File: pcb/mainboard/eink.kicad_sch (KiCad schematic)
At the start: 48 parts, among them J401 FH12-40S-0.5SH, U401 MAX17135

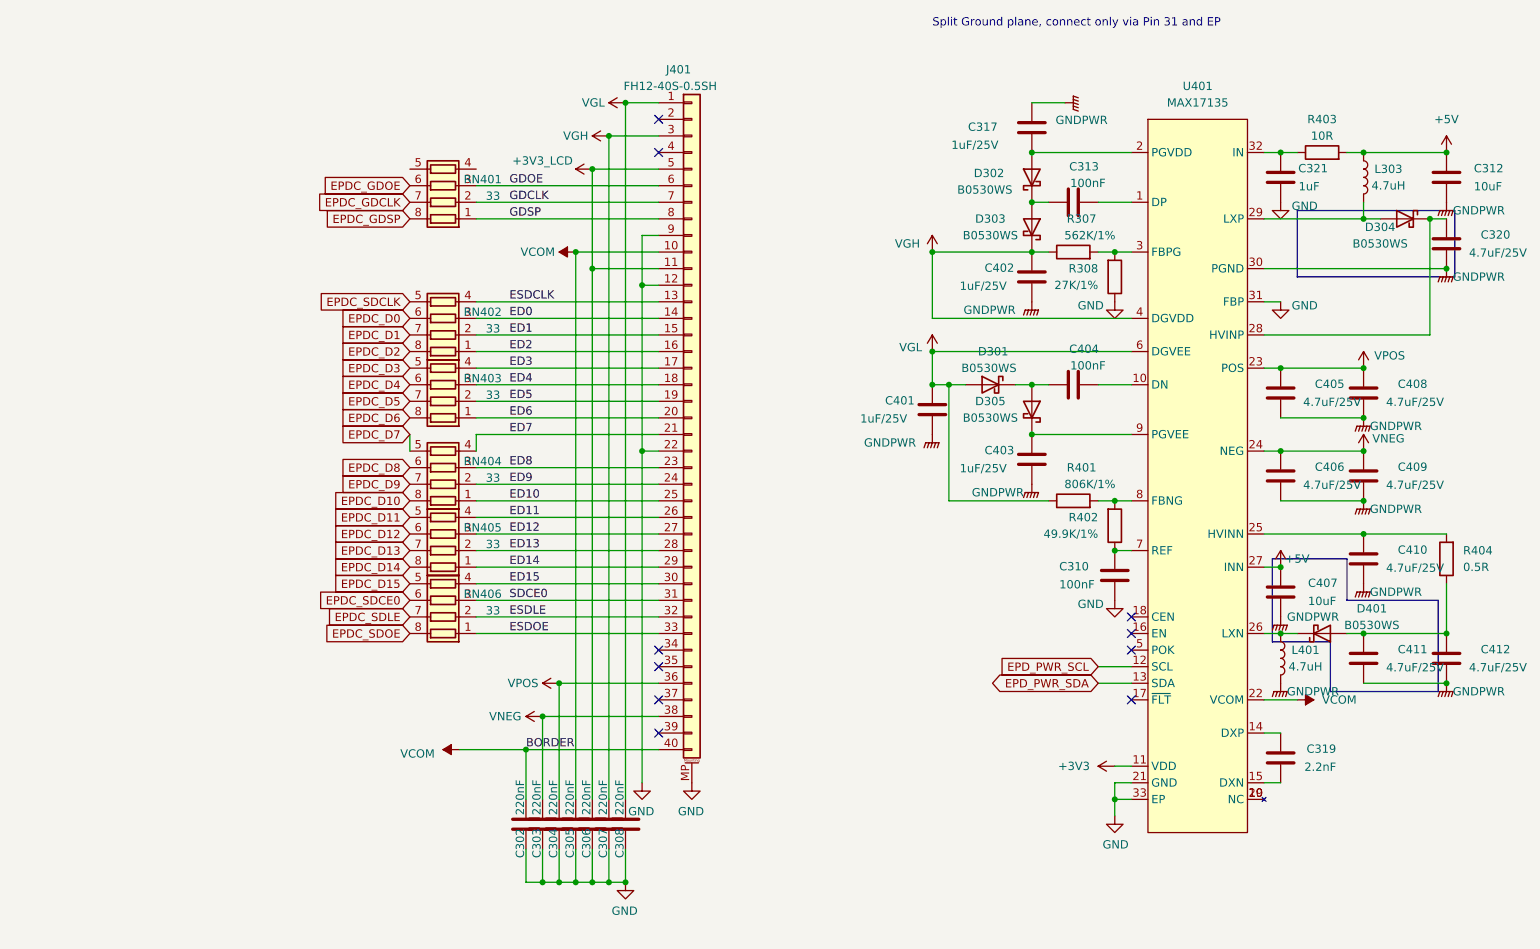
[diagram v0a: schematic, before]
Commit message: pcb: r0p4
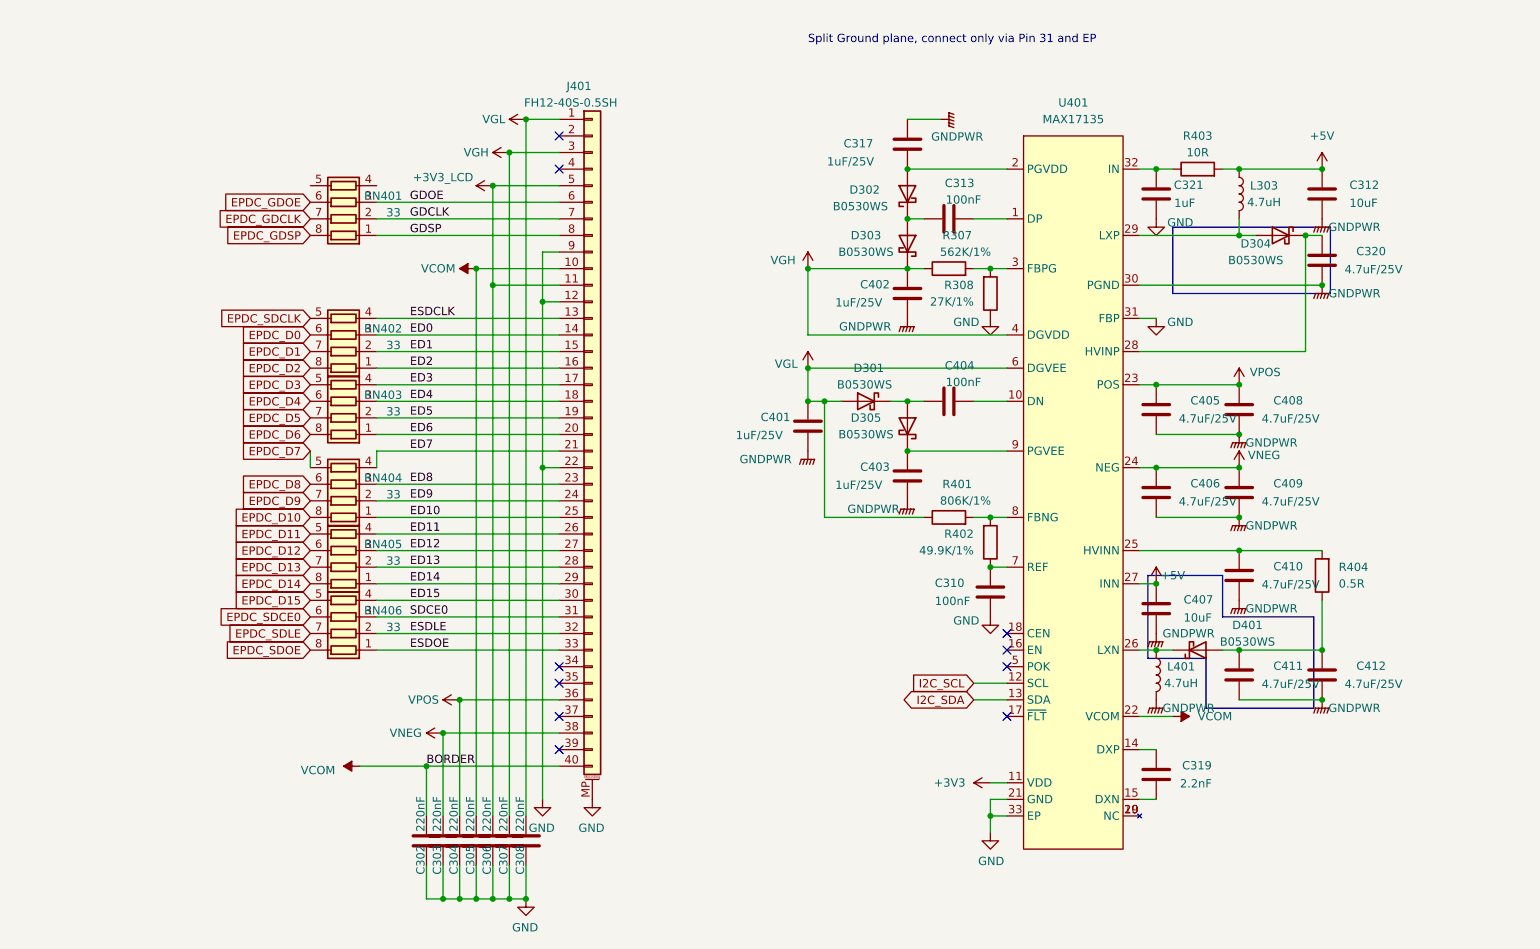
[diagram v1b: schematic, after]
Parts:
- L303, L401: footprint footprints:L_1212 -> footprints:L_FXL0420; LCSC C340379 -> C167208
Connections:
- net EPD_PWR_SCL renamed I2C_SCL
- net EPD_PWR_SDA renamed I2C_SDA
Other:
- company: Copyright 2021 Modos / Engineer: Wenting Zhang -> Copyright 2022 Modos / Engineer: Wenting Zhang
- moved on the sheet: C302, C303, C304, C305, C306, C307, C308, C310, C312, C313, C317, C319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

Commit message: pcb: r0p5
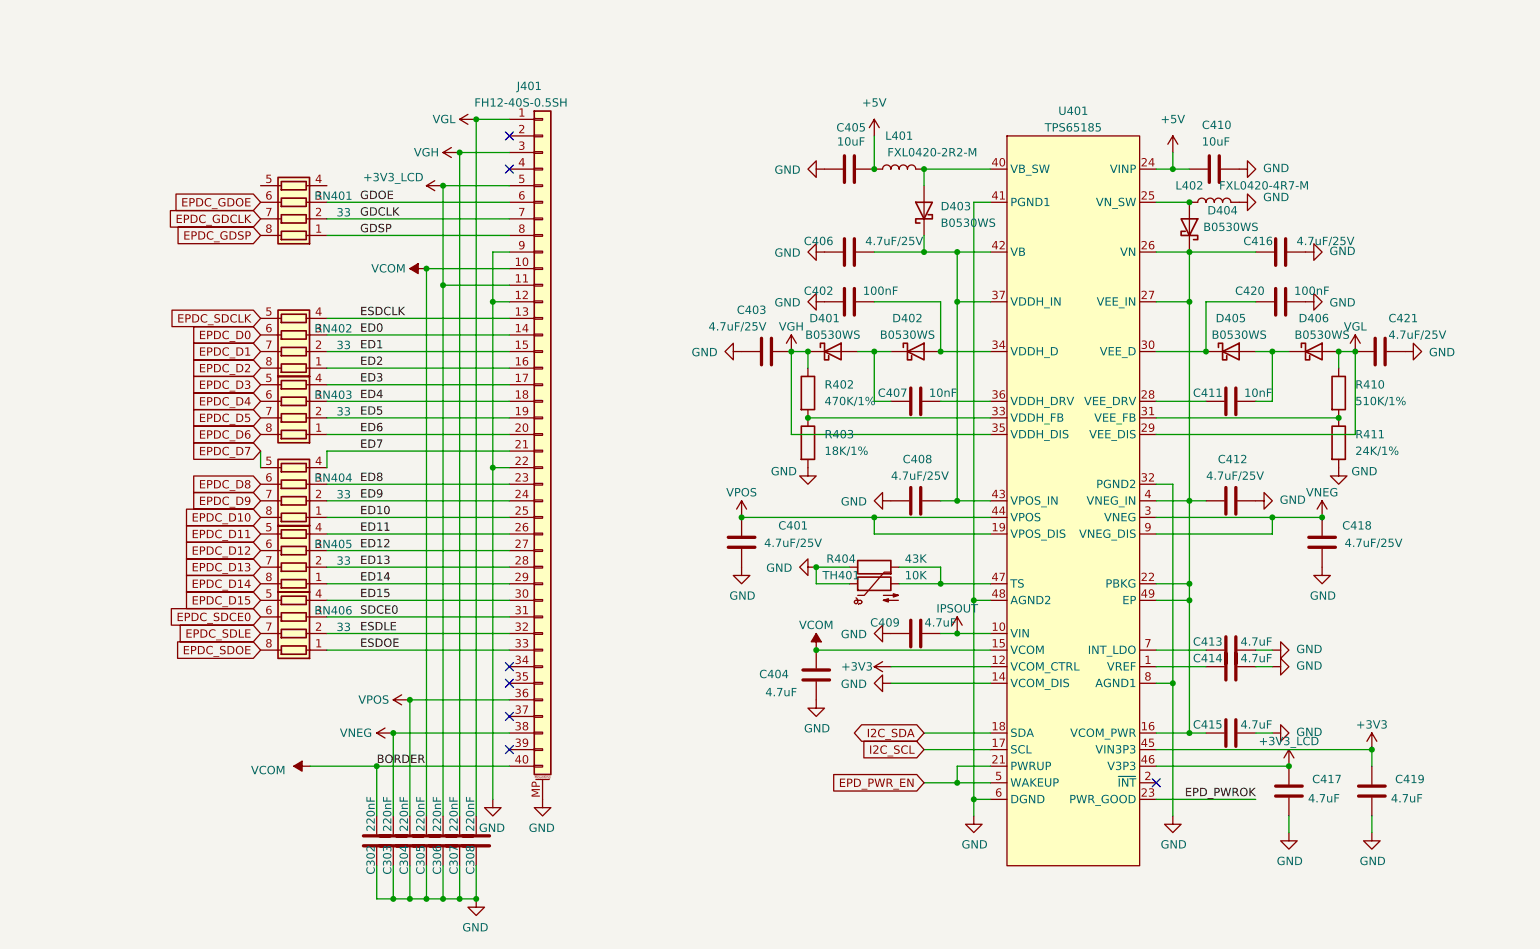
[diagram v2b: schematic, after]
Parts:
- removed C310, C313: 100nF, Capacitor_SMD:C_0402_1005Metric, symbol Device:C
- removed C312: 10uF, Capacitor_SMD:C_0603_1608Metric, symbol Device:C
- removed C317: 1uF/25V, Capacitor_SMD:C_0805_2012Metric, symbol Device:C
- removed C319: 2.2nF, Capacitor_SMD:C_0402_1005Metric, symbol Device:C
- removed C320: 4.7uF/25V, Capacitor_SMD:C_0805_2012Metric, symbol Device:C
- removed C321: 1uF, Capacitor_SMD:C_0402_1005Metric, symbol Device:C
- removed D301, D302, D303, D304, D305: B0530WS, Diode_SMD:D_SOD-323, symbol Device:D_Schottky
- removed L303: 4.7uH, footprints:L_FXL0420, symbol Device:L
- removed R307: 562K/1%, Resistor_SMD:R_0402_1005Metric, symbol Device:R
- removed R308: 27K/1%, Resistor_SMD:R_0402_1005Metric, symbol Device:R
- removed R401: 806K/1%, Resistor_SMD:R_0402_1005Metric, symbol Device:R
- removed U401: MAX17135, Package_DFN_QFN:QFN-32-1EP_5x5mm_P0.5mm_EP3.1x3.1mm_ThermalVias, symbol symbols:MAX17135
- added C413, C414, C415, C417, C419: 4.7uF, Capacitor_SMD:C_0603_1608Metric, symbol Device:C
- added C416, C418, C421: 4.7uF/25V, Capacitor_SMD:C_0805_2012Metric, symbol Device:C
- added C420: 100nF, Capacitor_SMD:C_0402_1005Metric, symbol Device:C
- added D402, D403, D404, D405, D406: B0530WS, Diode_SMD:D_SOD-323, symbol Device:D_Schottky
- added L402: FXL0420-4R7-M, footprints:L_FXL0420, symbol Device:L
- added R410: 510K/1%, Resistor_SMD:R_0402_1005Metric, symbol Device:R
- added R411: 24K/1%, Resistor_SMD:R_0402_1005Metric, symbol Device:R
- added TH401: 10K, Resistor_SMD:R_0402_1005Metric, symbol Device:Thermistor_NTC
- added U401: TPS65185, footprints:QFN-48-1EP_7x7mm_P0.5mm_EP4.1x4.1mm_ThermalVias, symbol symbols:TPS65185
- C401, C403: value 1uF/25V -> 4.7uF/25V; LCSC C111769 -> (none); Ref.Price 0.0174 -> (none)
- C402: value 1uF/25V -> 100nF; footprint Capacitor_SMD:C_0805_2012Metric -> Capacitor_SMD:C_0402_1005Metric; LCSC C111769 -> (none); Ref.Price 0.0174 -> (none)
- C404: value 100nF -> 4.7uF; footprint Capacitor_SMD:C_0402_1005Metric -> Capacitor_SMD:C_0603_1608Metric; LCSC C56392 -> (none); Ref.Price 0.0023 -> (none)
- C405, C410: value 4.7uF/25V -> 10uF; footprint Capacitor_SMD:C_0805_2012Metric -> Capacitor_SMD:C_0603_1608Metric; LCSC C105489 -> (none); Ref.Price 0.0271 -> (none)
- C406, C408, C412: LCSC C105489 -> (none); Ref.Price 0.0271 -> (none)
- C407: value 10uF -> 10nF; footprint Capacitor_SMD:C_0603_1608Metric -> Capacitor_SMD:C_0402_1005Metric; LCSC C105490 -> (none); Ref.Price 0.0165 -> (none)
- C409: value 4.7uF/25V -> 4.7uF; footprint Capacitor_SMD:C_0805_2012Metric -> Capacitor_SMD:C_0603_1608Metric; LCSC C105489 -> (none); Ref.Price 0.0271 -> (none)
- C411: value 4.7uF/25V -> 10nF; footprint Capacitor_SMD:C_0805_2012Metric -> Capacitor_SMD:C_0402_1005Metric; LCSC C105489 -> (none); Ref.Price 0.0271 -> (none)
- D401: LCSC C475612 -> (none); Ref.Price 0.0209 -> (none)
- L401: value 4.7uH -> FXL0420-2R2-M; LCSC C167208 -> (none); Ref.Price 0.0643 -> (none)
- R402: value 49.9K/1% -> 470K/1%; LCSC C137969 -> (none); Ref.Price 0.001 -> (none)
- R403: value 10R -> 18K/1%; LCSC C137925 -> (none); Ref.Price 0.0006 -> (none)
- R404: value 0.5R -> 43K; footprint Resistor_SMD:R_0603_1608Metric -> Resistor_SMD:R_0402_1005Metric; LCSC C45312 -> (none); Ref.Price 0.004 -> (none)
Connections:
- net +3V3: now also C419.1, U401.12 (VCOM_CTRL), U401.45 (VIN3P3)
- net +3V3_LCD: now also C417.1, U401.46 (V3P3)
- net +5V: now also C405.2, C410.1, L401.1, U401.24 (VINP); no longer C407.2, R403.2
- net GND: now also C401.1, C402.1, C403.1, C404.1, C405.1, C406.1, C408.1, C409.1, C410.2, C412.2, R403.2, R404.1, C413.2, C414.2, C415.2, C416.2, C417.2, C418.1, C419.2, C420.2, C421.1, L402.2, R411.2, TH401.1, U401.14 (VCOM_DIS), U401.32 (PGND2), U401.41 (PGND1), U401.48 (AGND2), U401.6 (DGND), U401.8 (AGND1)
- net I2C_SCL: now also U401.17 (SCL)
- net I2C_SDA: now also U401.18 (SDA)
- net VCOM: now also C404.2, U401.15 (VCOM)
- net VGH: now also C403.2, D401.1 (K), R402.1, U401.35 (VDDH_DIS); no longer C402.2
- net VGL: now also C421.2, D406.2 (A), R410.1, U401.29 (VEE_DIS); no longer C401.2
- net VNEG: now also C418.2, U401.3 (VNEG), U401.9 (VNEG_DIS); no longer C406.2, C409.2
- net VPOS: now also C401.2, U401.19 (VPOS_DIS), U401.44 (VPOS); no longer C405.2, C408.2
- net at R402.2: now also R403.1, U401.33 (VDDH_FB)
- net at R404.2: now also TH401.2, U401.47 (TS); no longer C410.2
- removed net GNDPWR: C401.1, C402.1, C403.1, C405.1, C406.1, C407.1, C408.1, C409.1, C410.1, C411.1, C412.1, L401.2
- new net: C412.1, C415.1, C416.1, D404.1 (K), U401.16 (VCOM_PWR), U401.22 (PBKG), U401.26 (VN), U401.27 (VEE_IN), U401.4 (VNEG_IN), U401.49 (EP)
- new net: D404.2 (A), L402.1, U401.25 (VN_SW)
- new net: C407.1, D401.2 (A), D402.1 (K)
- new net: C402.2, D402.2 (A), U401.34 (VDDH_D)
- new net: C406.2, C408.2, D403.1 (K), U401.37 (VDDH_IN), U401.42 (VB), U401.43 (VPOS_IN)
- new net: D403.2 (A), L401.2, U401.40 (VB_SW)
- new net: C411.1, U401.28 (VEE_DRV)
- new net: C411.2, D405.2 (A), D406.1 (K)
- new net: C414.1, U401.1 (VREF)
- new net: C420.1, D405.1 (K), U401.30 (VEE_D)
- new net: R410.2, R411.1, U401.31 (VEE_FB)
- new net: C407.2, U401.36 (VDDH_DRV)
- new net: C413.1, U401.7 (INT_LDO)
- new net EPD_PWROK: U401.23 (PWR_GOOD)
- new net EPD_PWR_EN: U401.21 (PWRUP), U401.5 (WAKEUP)
- new net IPSOUT: C409.2, U401.10 (VIN)
- no-connect marks 10 -> 7
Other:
- note removed: "Split Ground plane, connect only via Pin 31 and EP"
- moved on the sheet: C302, C303, C304, C305, C306, C307, C308, J401, RN401, RN402, RN403, RN404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

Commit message: pcb: r0p6
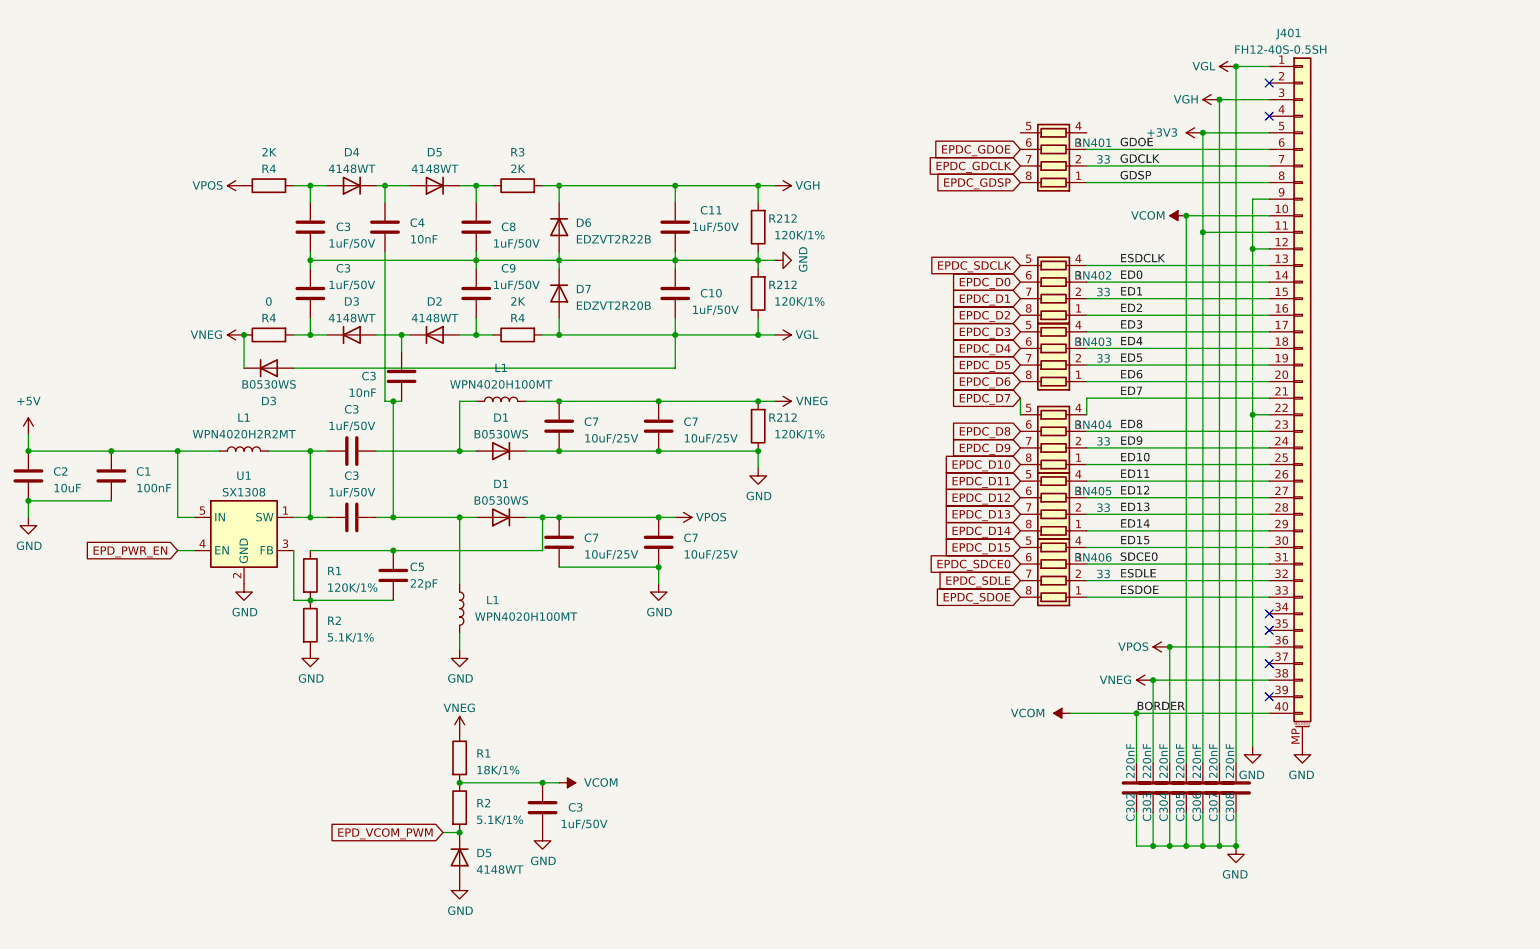
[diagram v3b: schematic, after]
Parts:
- removed C401, C403, C406, C408, C412, C416, C418, C421: 4.7uF/25V, Capacitor_SMD:C_0805_2012Metric, symbol Device:C
- removed C402, C420: 100nF, Capacitor_SMD:C_0402_1005Metric, symbol Device:C
- removed C404, C409, C413, C414, C415, C417, C419: 4.7uF, Capacitor_SMD:C_0603_1608Metric, symbol Device:C
- removed C405, C410: 10uF, Capacitor_SMD:C_0603_1608Metric, symbol Device:C
- removed C407, C411: 10nF, Capacitor_SMD:C_0402_1005Metric, symbol Device:C
- removed D401, D402, D403, D404, D405, D406: B0530WS, Diode_SMD:D_SOD-323, symbol Device:D_Schottky
- removed L401: FXL0420-2R2-M, footprints:L_FXL0420, symbol Device:L
- removed L402: FXL0420-4R7-M, footprints:L_FXL0420, symbol Device:L
- removed R402: 470K/1%, Resistor_SMD:R_0402_1005Metric, symbol Device:R
- removed R403: 18K/1%, Resistor_SMD:R_0402_1005Metric, symbol Device:R
- removed R404: 43K, Resistor_SMD:R_0402_1005Metric, symbol Device:R
- removed R410: 510K/1%, Resistor_SMD:R_0402_1005Metric, symbol Device:R
- removed R411: 24K/1%, Resistor_SMD:R_0402_1005Metric, symbol Device:R
- removed TH401: 10K, Resistor_SMD:R_0402_1005Metric, symbol Device:Thermistor_NTC
- removed U401: TPS65185, footprints:QFN-48-1EP_7x7mm_P0.5mm_EP4.1x4.1mm_ThermalVias, symbol symbols:TPS65185
- added C1: 100nF, Capacitor_SMD:C_0402_1005Metric, symbol Device:C
- added C10, C11, C3 (x5), C8, C9: 1uF/50V, Capacitor_SMD:C_0603_1608Metric, symbol Device:C
- added C2: 10uF, Capacitor_SMD:C_0603_1608Metric, symbol Device:C
- added C3, C4: 10nF, Capacitor_SMD:C_0402_1005Metric, symbol Device:C
- added C5: 22pF, Capacitor_SMD:C_0402_1005Metric, symbol Device:C
- added C7 (x4): 10uF/25V, Capacitor_SMD:C_0603_1608Metric, symbol Device:C
- added D1 (x2), D3: B0530WS, Diode_SMD:D_SOD-323, symbol Device:D
- added D2, D3, D4, D5 (x2): 4148WT, Diode_SMD:D_SOD-523, symbol Device:D
- added D6: EDZVT2R22B, Diode_SMD:D_SOD-323, symbol Device:D
- added D7: EDZVT2R20B, Diode_SMD:D_SOD-323, symbol Device:D
- added L1: WPN4020H2R2MT, Inductor_SMD:L_Changjiang_FNR4020S, symbol Device:L
- added L1 (x2): WPN4020H100MT, Inductor_SMD:L_Changjiang_FNR4020S, symbol Device:L
- added R1: 18K/1%, Resistor_SMD:R_0402_1005Metric, symbol Device:R
- added R1, R212 (x3): 120K/1%, Resistor_SMD:R_0402_1005Metric, symbol Device:R
- added R2 (x2): 5.1K/1%, Resistor_SMD:R_0402_1005Metric, symbol Device:R
- added R3, R4 (x2): 2K, Resistor_SMD:R_0402_1005Metric, symbol Device:R
- added R4: 0, Resistor_SMD:R_0402_1005Metric, symbol Device:R
- added U1: SX1308, Package_TO_SOT_SMD:SOT-23-6, symbol Regulator_Switching:MT3608
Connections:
- net +3V3_LCD is gone; now on net +3V3: C306.1, J401.11 (Pin_11), J401.5 (Pin_5)
- net +5V: now also C1.1, C2.1, L1.1, U1.5 (IN)
- net EPD_PWR_EN: now also U1.4 (EN)
- net GND: now also C1.2, C10.1, C11.2, C2.2, C3.1, C3.1, C3.2, C7.2, C7.2, C7.2, C7.2, C8.2, C9.1, D1.1 (K), D5.2 (A), D6.2 (A), D7.1 (K), L1.1, R2.2, R212.1, R212.1, R212.2, U1.2 (GND)
- net VCOM: now also C3.2, R1.2, R2.1
- net VGH: now also C11.1, D6.1 (K), R212.2, R3.2
- net VGL: now also C10.2, D3.2 (A), D7.2 (A), R212.1, R4.2
- net VNEG: now also C7.1, C7.1, D3.1 (K), L1.2, R1.1, R212.2, R4.1
- net VPOS: now also C5.2, C7.1, C7.1, D1.1 (K), R1.1, R4.1
- new net: C4.2, D4.1 (K), D5.2 (A)
- new net: C3.2, D4.2 (A), R4.2
- new net: C8.1, D5.1 (K), R3.1
- new net: C3.1, D2.1 (K), D3.2 (A)
- new net: C3.2, C3.2, C4.1, D1.2 (A), L1.2
- new net: C9.2, D2.2 (A), R4.1
- new net: C5.1, R1.2, R2.1, U1.3 (FB)
- new net: C3.1, D3.1 (K), R4.2
- new net: C3.1, C3.1, L1.2, U1.1 (SW)
- new net: C3.2, D1.2 (A), L1.1
- new net EPD_VCOM_PWM: D5.1 (K), R2.2
- no-connect marks 7 -> 6
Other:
- moved on the sheet: C302, C303, C304, C305, C306, C307, C308, J401, RN401, RN402, RN403, RN404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
